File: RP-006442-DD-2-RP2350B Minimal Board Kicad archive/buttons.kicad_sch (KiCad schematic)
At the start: 5 parts, among them SW10 SW_DIP_x08, SW11 SW_Omron_B3FS, SW12 SW_Omron_B3FS, SW13 SW_Omron_B3FS, SW14 SW_Omron_B3FS

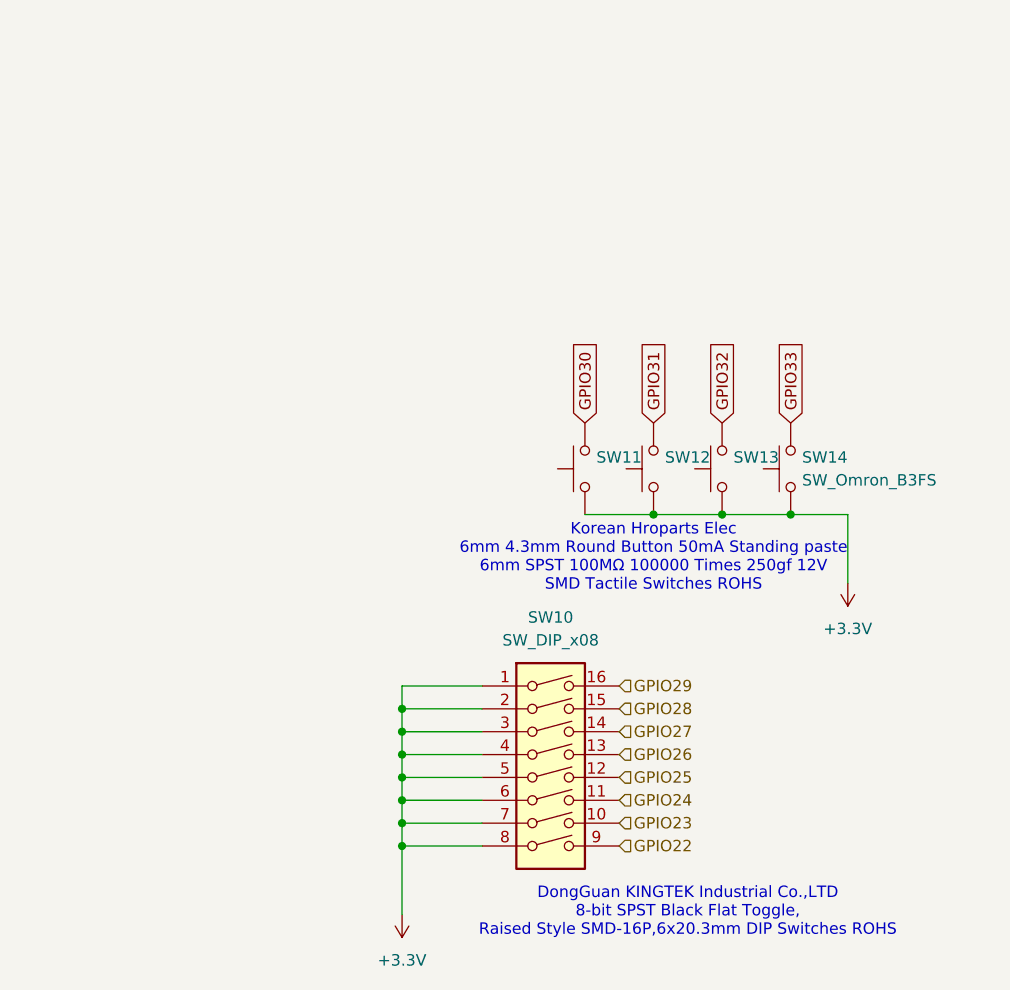
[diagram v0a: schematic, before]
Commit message: Update
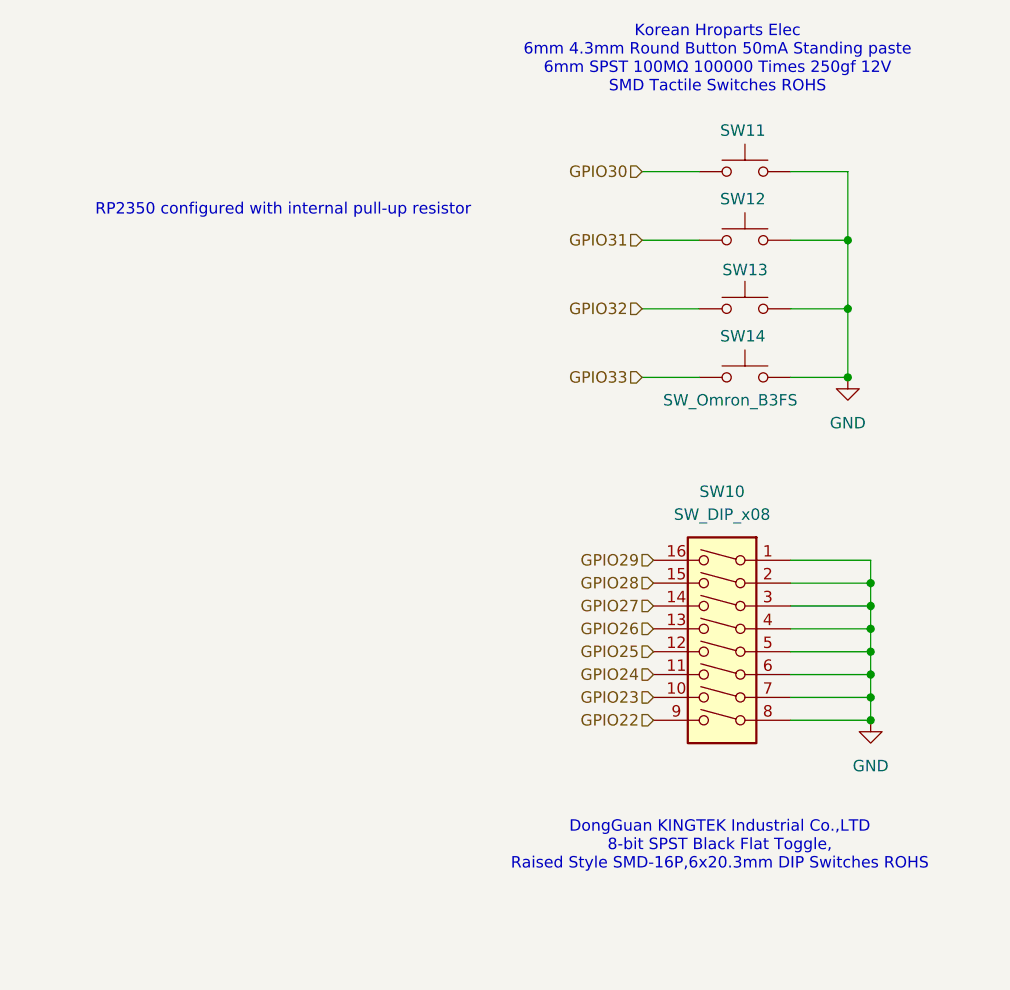
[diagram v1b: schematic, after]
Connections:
- net GPIO30: now also SW11.1; no longer SW11.2
- net GPIO31: now also SW12.1; no longer SW12.2
- net GPIO32: now also SW13.1; no longer SW13.2
- net GPIO33: now also SW14.1; no longer SW14.2
- net +3.3V renamed GND
- net GND: now also SW11.2, SW12.2, SW13.2, SW14.2; no longer SW11.1, SW12.1, SW13.1, SW14.1
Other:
- note added: "RP2350 configured with internal pull-up resistor"
- moved on the sheet: SW10, SW11, SW12, SW13, SW14
